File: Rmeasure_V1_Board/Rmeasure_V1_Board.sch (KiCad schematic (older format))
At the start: 52 parts, among them J1 USB_C_Receptacle_USB2.0, J2 CON_debug, J3 Conn_ARM_JTAG_SWD_10, J4 CON_CAN, J5 CON_CAN, SW1 BOOT, SW2 RST, U1 STM32F302C6Tx, U2 NCP1117-3.3_SOT223, U3 SN65HVD232, Y1 8MHz

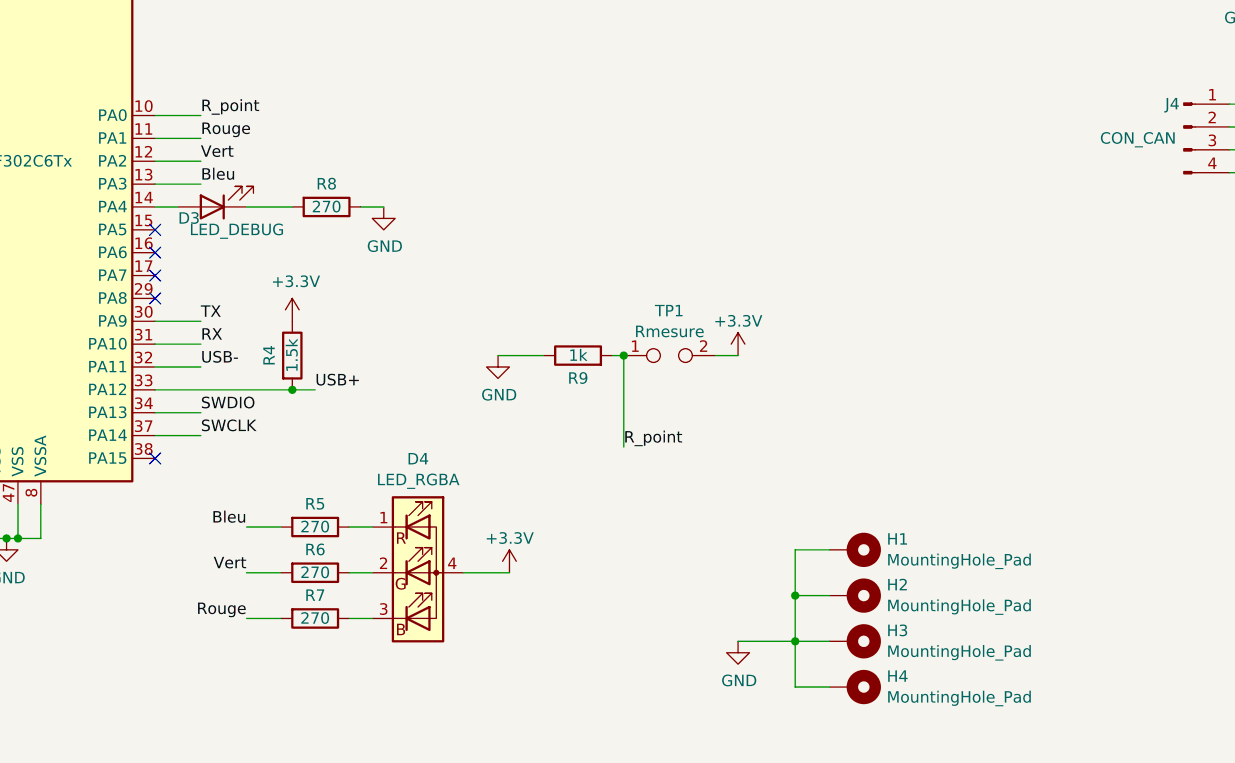
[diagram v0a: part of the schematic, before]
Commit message: ajout v3 carte alim
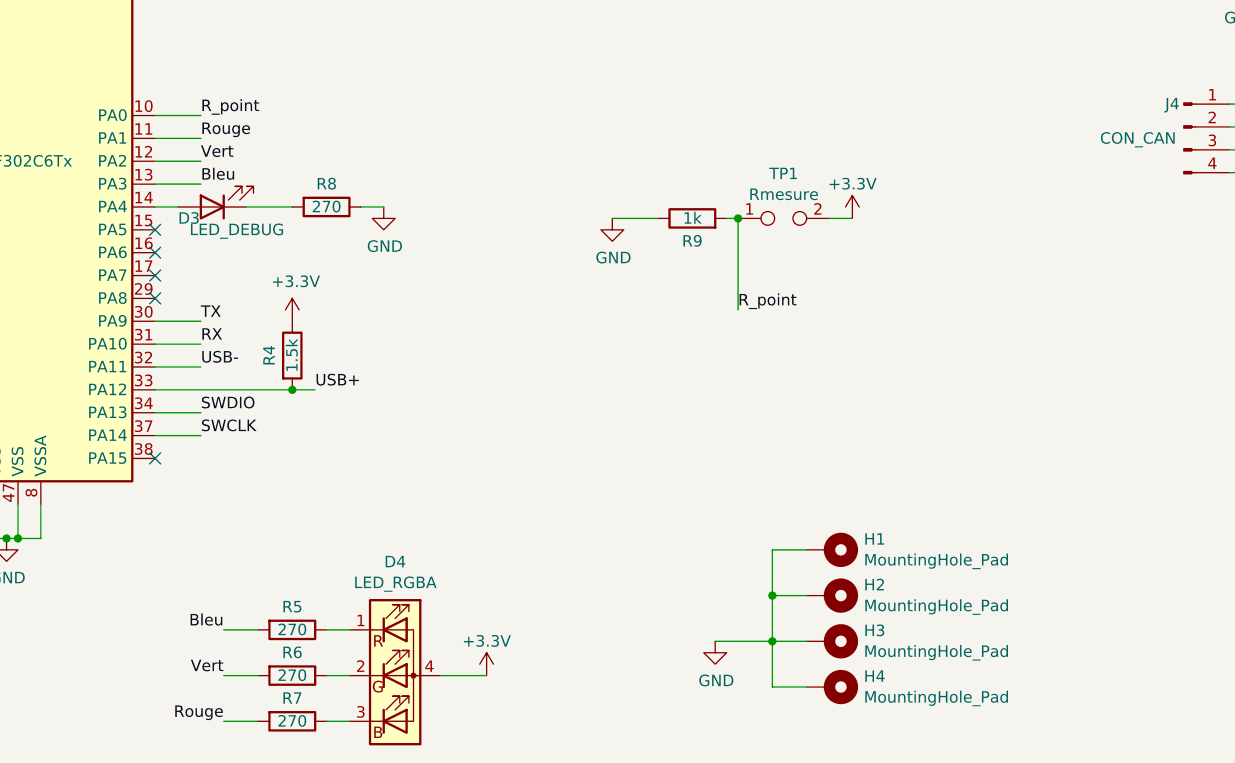
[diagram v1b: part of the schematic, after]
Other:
- moved on the sheet: D4, H1, H2, H3, H4, R5, R6, R7, R9, TP1
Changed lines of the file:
@@
 L Device:R R9
 U 1 1 617A6532
-P 5000 5750
-F 0 "R9" V 4900 5750 50  0000 C CNN
-F 1 "1k" V 5000 5750 50  0000 C CNN
-F 2 "Resistor_SMD:R_0805_2012Metric" V 4930 5750 50  0001 C CNN
-F 3 "~" H 5000 5750 50  0001 C CNN
-	1    5000 5750
+P 5500 5150
+F 0 "R9" V 5400 5150 50  0000 C CNN
+F 1 "1k" V 5500 5150 50  0000 C CNN
+F 2 "Resistor_SMD:R_0805_2012Metric" V 5430 5150 50  0001 C CNN
+F 3 "~" H 5500 5150 50  0001 C CNN
+	1    5500 5150
 	0    -1   -1   0
 $EndComp
@@
 L power:+3.3V #PWR027
 U 1 1 617A8FD6
-P 5700 5750
-F 0 "#PWR027" H 5700 5600 50  0001 C CNN
-F 1 "+3.3V" H 5700 5900 50  0000 C CNN
-F 2 "" H 5700 5750 50  0001 C CNN
-F 3 "" H 5700 5750 50  0001 C CNN
-	1    5700 5750
-	1    0    0    -1
-$EndComp
-Wire Wire Line
-	4650 5750 4850 5750
+P 6200 5150
+F 0 "#PWR027" H 6200 5000 50  0001 C CNN
+F 1 "+3.3V" H 6200 5300 50  0000 C CNN
+F 2 "" H 6200 5150 50  0001 C CNN
+F 3 "" H 6200 5150 50  0001 C CNN
+	1    6200 5150
+	1    0    0    -1
+$EndComp
+Wire Wire Line
+	5150 5150 5350 5150
 Wire Wire Line
 	3600 3700 4050 3700
 Wire Wire Line
-	5150 5750 5200 5750
+	5650 5150 5700 5150
 $Comp
 L Connector:TestPoint_2Pole TP1
 U 1 1 617B76A0
-P 5400 5750
-F 0 "TP1" H 5400 5945 50  0000 C CNN
-F 1 "Rmesure" H 5400 5854 50  0000 C CNN
-F 2 "TestPoint:TestPoint_Pad_4.0x4.0mm" H 5400 5750 50  0001 C CNN
-F 3 "~" H 5400 5750 50  0001 C CNN
-	1    5400 5750
-	1    0    0    -1
-$EndComp
-Wire Wire Line
-	5600 5750 5700 5750
+P 5900 5150
+F 0 "TP1" H 5900 5345 50  0000 C CNN
+F 1 "Rmesure" H 5900 5254 50  0000 C CNN
+F 2 "TestPoint:TestPoint_Pad_4.0x4.0mm" H 5900 5150 50  0001 C CNN
+F 3 "~" H 5900 5150 50  0001 C CNN
+	1    5900 5150
+	1    0    0    -1
+$EndComp
+Wire Wire Line
+	6100 5150 6200 5150
 $Comp
 L power:GND #PWR022
 U 1 1 617C164E
-P 4650 5750
-F 0 "#PWR022" H 4650 5500 50  0001 C CNN
-F 1 "GND" H 4655 5577 50  0000 C CNN
-F 2 "" H 4650 5750 50  0001 C CNN
-F 3 "" H 4650 5750 50  0001 C CNN
-	1    4650 5750
-	1    0    0    -1
-$EndComp
-Wire Wire Line
-	5200 5750 5200 6150
-Connection ~ 5200 5750
-Text Label 5200 6150 0    50   ~ 0
+P 5150 5150
+F 0 "#PWR022" H 5150 4900 50  0001 C CNN
+F 1 "GND" H 5155 4977 50  0000 C CNN
+F 2 "" H 5150 5150 50  0001 C CNN
+F 3 "" H 5150 5150 50  0001 C CNN
+	1    5150 5150
+	1    0    0    -1
+$EndComp
+Wire Wire Line
+	5700 5150 5700 5550
+Connection ~ 5700 5150
+Text Label 5700 5550 0    50   ~ 0
 R_point
 Wire Wire Line
@@
 L Device:R R5
 U 1 1 617EC642
-P 3850 6500
-F 0 "R5" V 3750 6500 50  0000 C CNN
-F 1 "270" V 3850 6500 50  0000 C CNN
-F 2 "Resistor_SMD:R_0805_2012Metric" V 3780 6500 50  0001 C CNN
-F 3 "~" H 3850 6500 50  0001 C CNN
-	1    3850 6500
+P 3750 6950
+F 0 "R5" V 3650 6950 50  0000 C CNN
+F 1 "270" V 3750 6950 50  0000 C CNN
+F 2 "Resistor_SMD:R_0805_2012Metric" V 3680 6950 50  0001 C CNN
+F 3 "~" H 3750 6950 50  0001 C CNN
+	1    3750 6950
 	0    1    1    0
 $EndComp
@@
 L Device:R R6
 U 1 1 617ED869
-P 3850 6700
-F 0 "R6" V 3750 6700 50  0000 C CNN
-F 1 "270" V 3850 6700 50  0000 C CNN
-F 2 "Resistor_SMD:R_0805_2012Metric" V 3780 6700 50  0001 C CNN
-F 3 "~" H 3850 6700 50  0001 C CNN
-	1    3850 6700
+P 3750 7150
+F 0 "R6" V 3650 7150 50  0000 C CNN
+F 1 "270" V 3750 7150 50  0000 C CNN
+F 2 "Resistor_SMD:R_0805_2012Metric" V 3680 7150 50  0001 C CNN
+F 3 "~" H 3750 7150 50  0001 C CNN
+	1    3750 7150
 	0    1    1    0
 $EndComp
@@
 L Device:R R7
 U 1 1 617EDE60
-P 3850 6900
-F 0 "R7" V 3750 6900 50  0000 C CNN
-F 1 "270" V 3850 6900 50  0000 C CNN
-F 2 "Resistor_SMD:R_0805_2012Metric" V 3780 6900 50  0001 C CNN
-F 3 "~" H 3850 6900 50  0001 C CNN
-	1    3850 6900
-	0    1    1    0
-$EndComp
-Wire Wire Line
-	4000 6500 4100 6500
-Wire Wire Line
-	4000 6700 4100 6700
-Wire Wire Line
-	4000 6900 4100 6900
-Wire Wire Line
-	3550 6500 3700 6500
-Wire Wire Line
-	3700 6700 3550 6700
-Wire Wire Line
-	3700 6900 3550 6900
-Text Label 3550 6900 2    50   ~ 0
+P 3750 7350
+F 0 "R7" V 3650 7350 50  0000 C CNN
+F 1 "270" V 3750 7350 50  0000 C CNN
+F 2 "Resistor_SMD:R_0805_2012Metric" V 3680 7350 50  0001 C CNN
+F 3 "~" H 3750 7350 50  0001 C CNN
+	1    3750 7350
+	0    1    1    0
+$EndComp
+Wire Wire Line
+	3900 6950 4000 6950
+Wire Wire Line
+	3900 7150 4000 7150
+Wire Wire Line
+	3900 7350 4000 7350
+Wire Wire Line
+	3450 6950 3600 6950
+Wire Wire Line
+	3600 7150 3450 7150
+Wire Wire Line
+	3600 7350 3450 7350
+Text Label 3450 7350 2    50   ~ 0
 Rouge
-Text Label 3550 6700 2    50   ~ 0
+Text Label 3450 7150 2    50   ~ 0
 Vert
-Text Label 3550 6500 2    50   ~ 0
+Text Label 3450 6950 2    50   ~ 0
 Bleu
 Wire Wire Line
-	4500 6700 4700 6700
+	4400 7150 4600 7150
 $Comp
 L Device:LED_RGBA D4
 U 1 1 61698EB2
-P 4300 6700
-F 0 "D4" H 4300 7197 50  0000 C CNN
-F 1 "LED_RGBA" H 4300 7106 50  0000 C CNN
-F 2 "LED_SMD:LED_SK6812_EC15_1.5x1.5mm" H 4300 6650 50  0001 C CNN
-F 3 "~" H 4300 6650 50  0001 C CNN
-	1    4300 6700
+P 4200 7150
+F 0 "D4" H 4200 7647 50  0000 C CNN
+F 1 "LED_RGBA" H 4200 7556 50  0000 C CNN
+F 2 "LED_SMD:LED_SK6812_EC15_1.5x1.5mm" H 4200 7100 50  0001 C CNN
+F 3 "~" H 4200 7100 50  0001 C CNN
+	1    4200 7150
 	1    0    0    -1
 $EndComp
@@
 L power:+3.3V #PWR023
 U 1 1 61699C32
-P 4700 6700
-F 0 "#PWR023" H 4700 6550 50  0001 C CNN
-F 1 "+3.3V" H 4700 6850 50  0000 C CNN
-F 2 "" H 4700 6700 50  0001 C CNN
-F 3 "" H 4700 6700 50  0001 C CNN
-	1    4700 6700
+P 4600 7150
+F 0 "#PWR023" H 4600 7000 50  0001 C CNN
+F 1 "+3.3V" H 4600 7300 50  0000 C CNN
+F 2 "" H 4600 7150 50  0001 C CNN
+F 3 "" H 4600 7150 50  0001 C CNN
+	1    4600 7150
 	1    0    0    -1
 $EndComp
@@
 L Mechanical:MountingHole_Pad H1
 U 1 1 616ACCC9
-P 6200 6600
-F 0 "H1" V 6154 6750 50  0000 L CNN
-F 1 "MountingHole_Pad" V 6245 6750 50  0000 L CNN
-F 2 "MountingHole:MountingHole_3.2mm_M3_Pad_Via" H 6200 6600 50  0001 C CNN
-F 3 "~" H 6200 6600 50  0001 C CNN
-	1    6200 6600
+P 6100 6600
+F 0 "H1" V 6054 6750 50  0000 L CNN
+F 1 "MountingHole_Pad" V 6145 6750 50  0000 L CNN
+F 2 "MountingHole:MountingHole_3.2mm_M3_Pad_Via" H 6100 6600 50  0001 C CNN
+F 3 "~" H 6100 6600 50  0001 C CNN
+	1    6100 6600
 	0    1    1    0
 $EndComp
@@
 L Mechanical:MountingHole_Pad H2
 U 1 1 616ADA50
-P 6200 6800
-F 0 "H2" V 6154 6950 50  0000 L CNN
-F 1 "MountingHole_Pad" V 6245 6950 50  0000 L CNN
-F 2 "MountingHole:MountingHole_3.2mm_M3_Pad_Via" H 6200 6800 50  0001 C CNN
-F 3 "~" H 6200 6800 50  0001 C CNN
-	1    6200 6800
+P 6100 6800
+F 0 "H2" V 6054 6950 50  0000 L CNN
+F 1 "MountingHole_Pad" V 6145 6950 50  0000 L CNN
+F 2 "MountingHole:MountingHole_3.2mm_M3_Pad_Via" H 6100 6800 50  0001 C CNN
+F 3 "~" H 6100 6800 50  0001 C CNN
+	1    6100 6800
 	0    1    1    0
 $EndComp
@@
 L Mechanical:MountingHole_Pad H3
 U 1 1 616ADFFD
-P 6200 7000
-F 0 "H3" V 6154 7150 50  0000 L CNN
-F 1 "MountingHole_Pad" V 6245 7150 50  0000 L CNN
-F 2 "MountingHole:MountingHole_3.2mm_M3_Pad_Via" H 6200 7000 50  0001 C CNN
-F 3 "~" H 6200 7000 50  0001 C CNN
-	1    6200 7000
+P 6100 7000
+F 0 "H3" V 6054 7150 50  0000 L CNN
+F 1 "MountingHole_Pad" V 6145 7150 50  0000 L CNN
+F 2 "MountingHole:MountingHole_3.2mm_M3_Pad_Via" H 6100 7000 50  0001 C CNN
+F 3 "~" H 6100 7000 50  0001 C CNN
+	1    6100 7000
 	0    1    1    0
 $EndComp
@@
 L Mechanical:MountingHole_Pad H4
 U 1 1 616AE5C5
-P 6200 7200
-F 0 "H4" V 6154 7350 50  0000 L CNN
-F 1 "MountingHole_Pad" V 6245 7350 50  0000 L CNN
-F 2 "MountingHole:MountingHole_3.2mm_M3_Pad_Via" H 6200 7200 50  0001 C CNN
-F 3 "~" H 6200 7200 50  0001 C CNN
-	1    6200 7200
+P 6100 7200
+F 0 "H4" V 6054 7350 50  0000 L CNN
+F 1 "MountingHole_Pad" V 6145 7350 50  0000 L CNN
+F 2 "MountingHole:MountingHole_3.2mm_M3_Pad_Via" H 6100 7200 50  0001 C CNN
+F 3 "~" H 6100 7200 50  0001 C CNN
+	1    6100 7200
 	0    1    1    0
 $EndComp
@@
 L power:GND #PWR040
 U 1 1 616AEB46
-P 5700 7000
-F 0 "#PWR040" H 5700 6750 50  0001 C CNN
-F 1 "GND" H 5705 6827 50  0000 C CNN
-F 2 "" H 5700 7000 50  0001 C CNN
-F 3 "" H 5700 7000 50  0001 C CNN
-	1    5700 7000
-	1    0    0    -1
-$EndComp
-Wire Wire Line
-	6100 6600 5950 6600
-Wire Wire Line
-	5950 6600 5950 6800
-Wire Wire Line
-	5950 7200 6100 7200
-Wire Wire Line
-	6100 7000 5950 7000
-Connection ~ 5950 7000
-Wire Wire Line
-	5950 7000 5950 7200
-Wire Wire Line
-	6100 6800 5950 6800
-Connection ~ 5950 6800
-Wire Wire Line
-	5950 6800 5950 7000
-Wire Wire Line
-	5950 7000 5700 7000
+P 5600 7000
+F 0 "#PWR040" H 5600 6750 50  0001 C CNN
+F 1 "GND" H 5605 6827 50  0000 C CNN
+F 2 "" H 5600 7000 50  0001 C CNN
+F 3 "" H 5600 7000 50  0001 C CNN
+	1    5600 7000
+	1    0    0    -1
+$EndComp
+Wire Wire Line
+	6000 6600 5850 6600
+Wire Wire Line
+	5850 6600 5850 6800
+Wire Wire Line
+	5850 7200 6000 7200
+Wire Wire Line
+	6000 7000 5850 7000
+Connection ~ 5850 7000
+Wire Wire Line
+	5850 7000 5850 7200
+Wire Wire Line
+	6000 6800 5850 6800
+Connection ~ 5850 6800
+Wire Wire Line
+	5850 6800 5850 7000
+Wire Wire Line
+	5850 7000 5600 7000
 $Comp
 L Connector:USB_C_Receptacle_USB2.0 J1
